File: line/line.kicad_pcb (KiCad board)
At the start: 2 copper layers, 75 x 75 mm, 41 parts, among them J1 MAINS, J2 CONTROL, Q1 Q_NMOS_GDS, Q2 Q_NMOS_GDS, U1 LM324, U2 LTV-817S

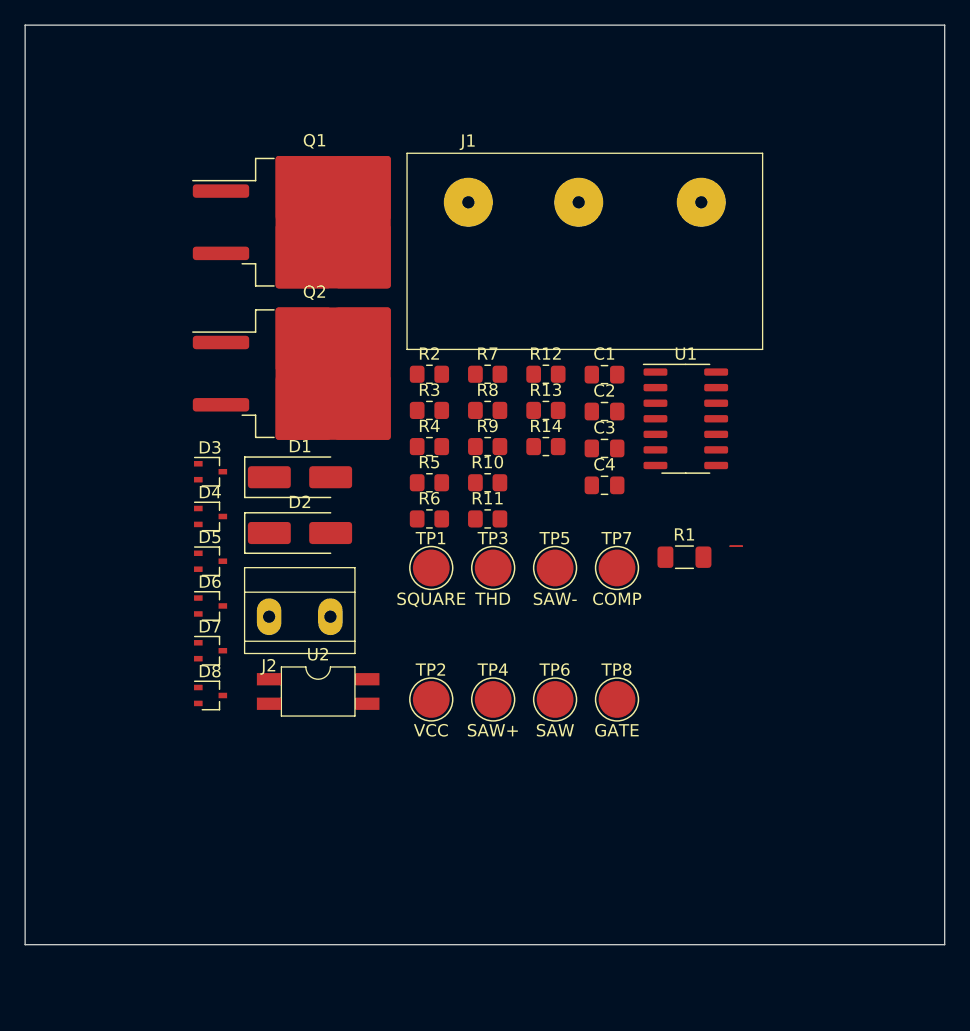
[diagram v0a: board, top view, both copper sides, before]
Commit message: WIP
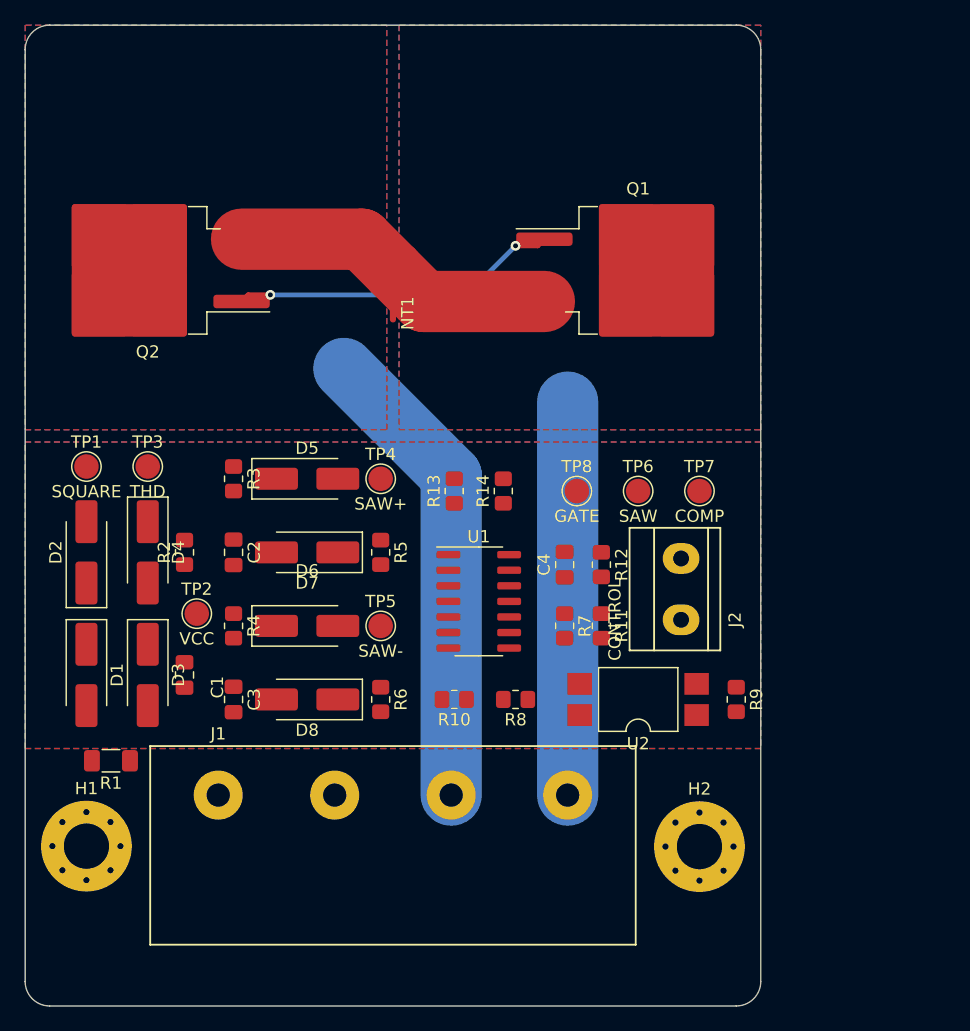
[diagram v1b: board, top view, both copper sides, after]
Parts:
- added H1: MountingHole, MountingHole:MountingHole_3.7mm_Pad_Via, F.Cu at (105.0, 137.0)
- added H2: MountingHole, MountingHole:MountingHole_3.7mm_Pad_Via, F.Cu at (155.0, 137.0)
- D3, D4, D5, D6, D7, D8: value BAT54W -> SS13A; footprint Package_TO_SOT_SMD:SOT-323_SC-70 -> Diode_SMD:D_SMA_Handsoldering
- J1: footprint Drake:HB-9500-3P -> Drake:HB-9500-4P
- NT1: footprint NetTie:NetTie-2_THT_Pad0.3mm -> NetTie:NetTie-2_SMD_Pad0.5mm
- Q1, Q2: value Q_NMOS_GDS -> WMM38N60C2
- R14: value 270??? -> 3R9
- TP1, TP2, TP3, TP4, TP5, TP6, TP7, TP8: footprint TestPoint:TestPoint_Pad_D3.0mm -> TestPoint:TestPoint_Pad_D2.0mm
- moved J1 52.5 mm to (115.8, 132.8)
- moved R1 49.6 mm to (107.0, 130.0), turned to 180 degrees
- moved C1 42.1 mm to (113.0, 123.0), turned to -90 degrees
- moved C3 36.5 mm to (117.0, 125.0), turned to -90 degrees
- moved J2 33.6 mm to (153.5, 118.5), turned to 90 degrees
- moved NT1 33.4 mm to (130.0, 93.5), turned to -90 degrees
- moved C2 32.4 mm to (117.0, 113.0), turned to -90 degrees
- moved TP3 29.4 mm to (110.0, 106.0)
- moved TP1 29.3 mm to (105.0, 106.0)
- moved R9 28.9 mm to (158.0, 125.0), turned to -90 degrees
- moved Q1 26.7 mm to (150.0, 90.0)
- moved U2 26.1 mm to (150.0, 125.0), turned to 180 degrees
- moved R2 24.7 mm to (113.0, 113.0), turned to 90 degrees
- moved D1 23.7 mm to (105.0, 123.0), turned to -90 degrees
- moved R8 23.7 mm to (140.0, 125.0), turned to 180 degrees
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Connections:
- D3 pad 1: Net-(D1-K) -> VCC
- D3 pad 2: unconnected-(D3-NC-Pad2) -> Net-(D1-K)
- D4 pad 1: Net-(D4-A) -> GND
- D4 pad 2: unconnected-(D4-NC-Pad2) -> Net-(D4-A)
- D5 pad 1: Net-(D5-A) -> Net-(D5-K)
- D5 pad 2: unconnected-(D5-NC-Pad2) -> Net-(D5-A)
- D6 pad 1: Net-(D6-A) -> Net-(D6-K)
- D6 pad 2: unconnected-(D6-NC-Pad2) -> Net-(D6-A)
- D7 pad 1: GND -> Net-(D5-A)
- D7 pad 2: unconnected-(D7-NC-Pad2) -> GND
- D8 pad 1: GND -> Net-(D6-A)
- D8 pad 2: unconnected-(D8-NC-Pad2) -> GND
- J1 pad 2: /MAINS_L_IN -> /MAINS_N
- J1 pad 3: /MAINS_L_OUT -> /MAINS_L_IN
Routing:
- net /MAINS_L_IN: track 0.00 -> 38.4 mm
- net /MAINS_L_OUT: track 0.00 -> 32.1 mm
- net Net-(Q1-G): track 0.00 -> 26.8 mm, vias 0 -> 2
- net /S2S: track 0.00 -> 26.8 mm
- added copper zone on B.Cu, net /MAINS_L_IN
- added copper zone on F.Cu, net /MAINS_L_IN
- added copper zone on B.Cu, net /MAINS_L_OUT
- added copper zone on F.Cu, net /MAINS_L_OUT
- added copper zone on B.Cu, net GND
- added copper zone on F.Cu, net GND
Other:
- board size 75 x 75 mm -> 60 x 80 mm
